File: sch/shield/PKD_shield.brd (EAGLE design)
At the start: 68.6 x 53.3 mm, 35 parts, among them IC1 LM393N, IC2 TL084P, IC3 PIC12F683P, IC5 74HCT243N, Q1 BS170

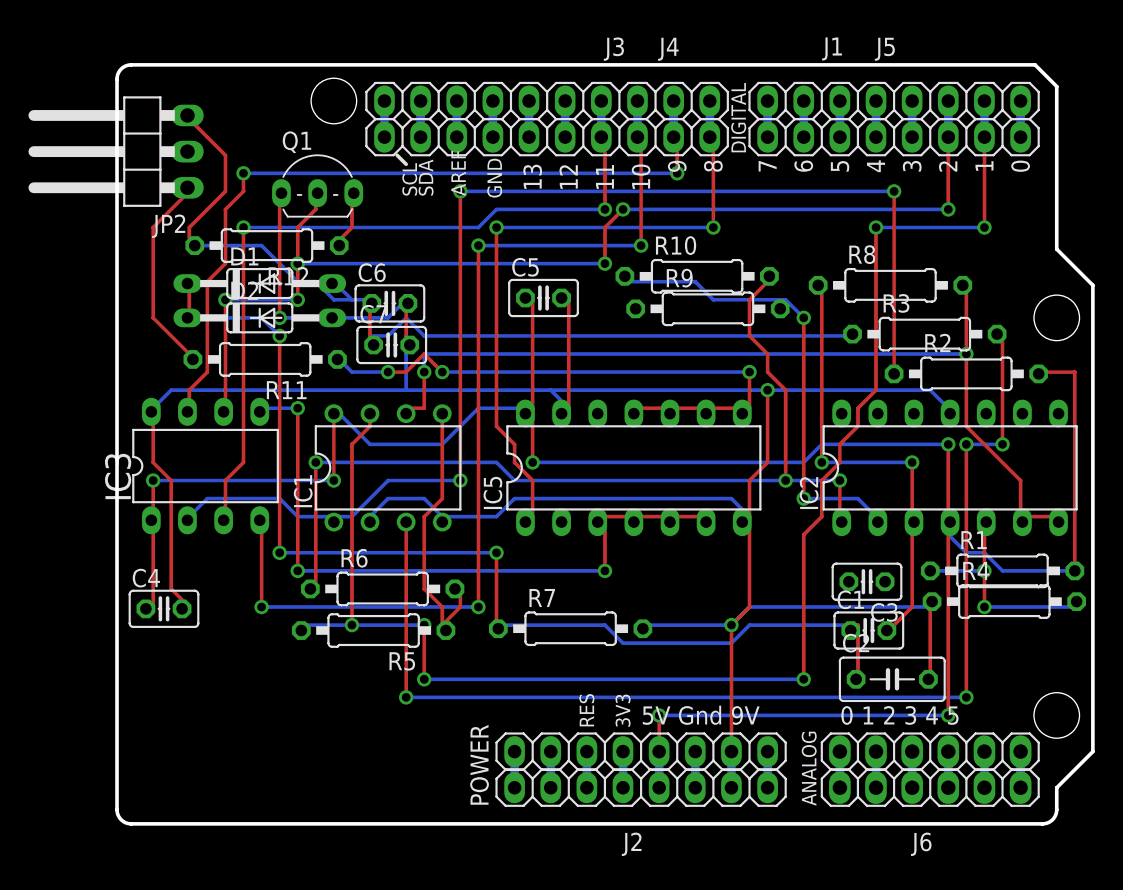
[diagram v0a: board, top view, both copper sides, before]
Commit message: Minor update
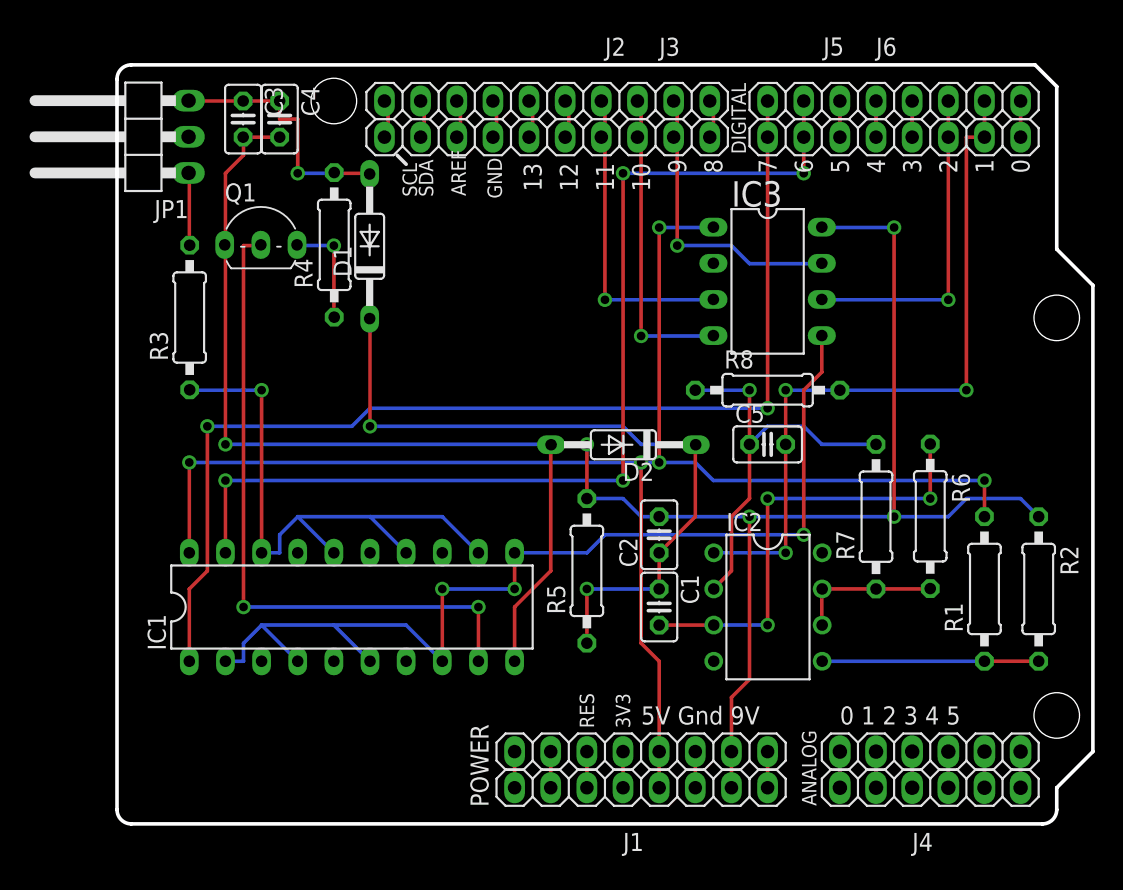
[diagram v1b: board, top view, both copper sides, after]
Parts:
- removed C6: 1n, rcl:C025-025X050
- removed C7: 2n2, rcl:C025-025X050
- removed IC5: 74HCT243N, 74xx-eu:DIL14
- removed JP2: (no value), pinhead:1X03/90
- removed R10: 100k, rcl:0207/10
- removed R11: 33, rcl:0207/10
- removed R12: 220, rcl:0207/10
- removed R9: 10k, rcl:0207/10
- added JP1: (no value), pinhead:1X03/90
- C2: device rcl:C050-030X075 -> rcl:C025-025X050
- C3: value 100p -> 1n
- C4: value 33n -> 2n2
- C5: value 33n -> 100p
- IC1: value LM393N -> 74HC244N; device linear:DIL08 -> 74xx-eu:DIL20
- IC2: value TL084P -> TL082P; device linear:DIL14 -> linear:DIL08
- J2: device SmartPrj:1X08-TH -> SmartPrj:1X10-TH
- J4: device SmartPrj:1X10-TH -> pinhead:1X06
- J6: device pinhead:1X06 -> SmartPrj:1X08-TH
- R2: value 10k -> 100k
- R3: value 240k -> 33
- R4: value 100k -> 220
- R5: value 10k -> 510k
- R6: value 2,2k -> 100k
- R7: value 510k -> 10k
- moved C3 54.6 mm to (8.86, 49.5), turned to 270 degrees
- moved R4 53.3 mm to (15.3, 40.7), turned to 90 degrees
- moved R3 51.7 mm to (5.11, 35.6), turned to 90 degrees
- moved J1 51.4 mm to (36.8, 2.54), turned to 0 degrees
- moved J4 50.9 mm to (57.1, 5.08), turned to 0 degrees
- moved J2 48.7 mm to (30.2, 50.8), turned to 180 degrees
- moved J6 43.3 mm to (54.6, 48.3), turned to 180 degrees
- moved IC3 41.6 mm to (45.7, 38.1), turned to 270 degrees
- moved R6 38.8 mm to (57.1, 21.6), turned to 270 degrees
- moved C4 35.4 mm to (11.4, 49.5), turned to 270 degrees
- moved D2 27.1 mm to (35.6, 26.6), turned to 180 degrees
- moved R7 22.9 mm to (53.3, 21.6), turned to 90 degrees
- moved C2 19.3 mm to (38.1, 20.3), turned to 90 degrees
- moved C5 18.8 mm to (45.7, 26.7)
- moved IC2 16.1 mm to (45.7, 15.2), turned to 270 degrees
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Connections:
- removed net CROSS_LO: IC1.1, IC3.2, R2.1
- removed net LO_PKD_U: C3.2, IC2.1, R10.2, R6.1
- removed net N$14: J1.7, J5.7
- removed net N$15: J1.8, J5.8
- removed net N$28: IC1.3, R3.2
- removed net N$35: IC1.5, R5.1, R6.2
- new net N$2: IC1.9, Q1.2
- new net N$5: J2.1, J3.1
- new net PWR_OE2: IC1.19, J5.7, J6.7
- new net V+: IC2.8
- new net V-: IC2.4
- net +9V: now also J1.8; no longer J2.8
- net ANT_LO: now also C3.1, C4.1, JP1.3, R4.2; no longer C6.1, C7.1, JP2.3, R12.2, R3.1
- net BIT_IN: now also J2.4; no longer J4.4
- net GND: now also C3.2, IC1.10, J1.7, R2.1, R5.2; no longer C5.2, C6.2, C7.2, IC1.2, IC1.4, IC2.11, IC5.13, IC5.7, J2.7, R4.1, R7.2
- net LO_PKD: now also C5.2, IC2.1, J6.2, R8.2; no longer IC1.7, J1.2, R5.2
- net N$1: now also J1.3; no longer J2.3
- net N$11: now also J6.4; no longer J1.4
- net N$12: now also J6.5; no longer J1.5
- net N$13: now also J6.6; no longer J1.6
- net N$141: now also J2.9; no longer J4.9
- net N$142: now also J2.10; no longer J4.10
- net N$16: now also R2.2; no longer R4.2
- net N$17: now also R5.1; no longer R7.1
- net N$18: now also J4.1; no longer J6.1
- net N$19: now also J4.2; no longer J6.2
- net N$20: now also J4.3; no longer J6.3
- net N$21: now also J4.4; no longer J6.4
- net N$22: now also J4.5; no longer J6.5
- net N$222: now also J2.8; no longer J4.8
- net N$223: now also J1.4; no longer J2.4
- net N$23: now also J4.6; no longer J6.6
- net N$24: now also J2.7; no longer J4.7
- net N$25: now also J1.6; no longer J2.6
- net N$26: now also R6.1; no longer R8.1
- net N$27: now also C5.1, R7.2, R8.1; no longer C3.1, R10.1, R9.2
- net N$29: now also JP1.1, R3.2; no longer JP2.1, R11.2
- net N$3: now also J2.6; no longer J4.6
- net N$30: now also IC1.12, IC1.14, IC1.16, IC1.18, R3.1; no longer IC5.10, IC5.11, IC5.8, IC5.9, R11.1
- net N$31: now also J1.2; no longer J2.2
- net N$32: now also J1.1; no longer J2.1
- net N$34: now also R4.1; no longer R12.1
- net N$4: now also J2.5; no longer J4.5
- net N$8: now also J6.1; no longer J1.1
- net NRST: now also J2.3; no longer J4.3
- net OCLK: now also J6.3; no longer J1.3, Q1.2
- net PWR_LO: now also IC1.11, IC1.2, IC1.4, IC1.6, IC1.8; no longer IC5.3, IC5.4, IC5.5, IC5.6
- net PWR_OE1: now also IC1.1, J5.8, J6.8; no longer IC5.1, J3.1, J4.1
- net R/E: now also J2.2; no longer J4.2
- net VCC: now also IC1.20, J1.5; no longer C4.1, C5.1, IC1.8, IC2.4, IC5.14, J2.5, R2.2
- net VMID: now also R6.2, R7.1; no longer IC1.6, R8.2, R9.1
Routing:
- net CROSS_LO: track 85.8 -> 0.00 mm, vias 3 -> 0
- net N$28: track 80.8 -> 0.00 mm, vias 4 -> 0
- net PWR_OE2: track 0.00 -> 72.4 mm, vias 0 -> 4
- net LO_PKD_U: track 65.5 -> 0.00 mm, vias 3 -> 0
- net VMID: track 65.8 -> 10.2 mm, vias 2 -> 0
- net LO_PKD: track 106.3 -> 50.8 mm, vias 6 -> 3
- net OCLK: track 77.7 -> 22.9 mm, vias 6 -> 1
- net VCC: track 160.1 -> 109.0 mm, vias 6 -> 5
- net ANT_LO: track 68.5 -> 18.0 mm, vias 0 -> 1
- net GND: track 198.4 -> 148.7 mm, vias 3 -> 5
- net N$2: track 0.00 -> 47.1 mm, vias 0 -> 2
- net NRST: track 69.1 -> 22.1 mm, vias 4 -> 1
- net R/E: track 54.2 -> 21.4 mm, vias 2 -> 1
- net BIT_IN: track 54.9 -> 22.1 mm, vias 2 -> 1
- net PWR_OE1: track 46.4 -> 78.5 mm
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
